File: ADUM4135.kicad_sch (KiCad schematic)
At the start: 24 parts

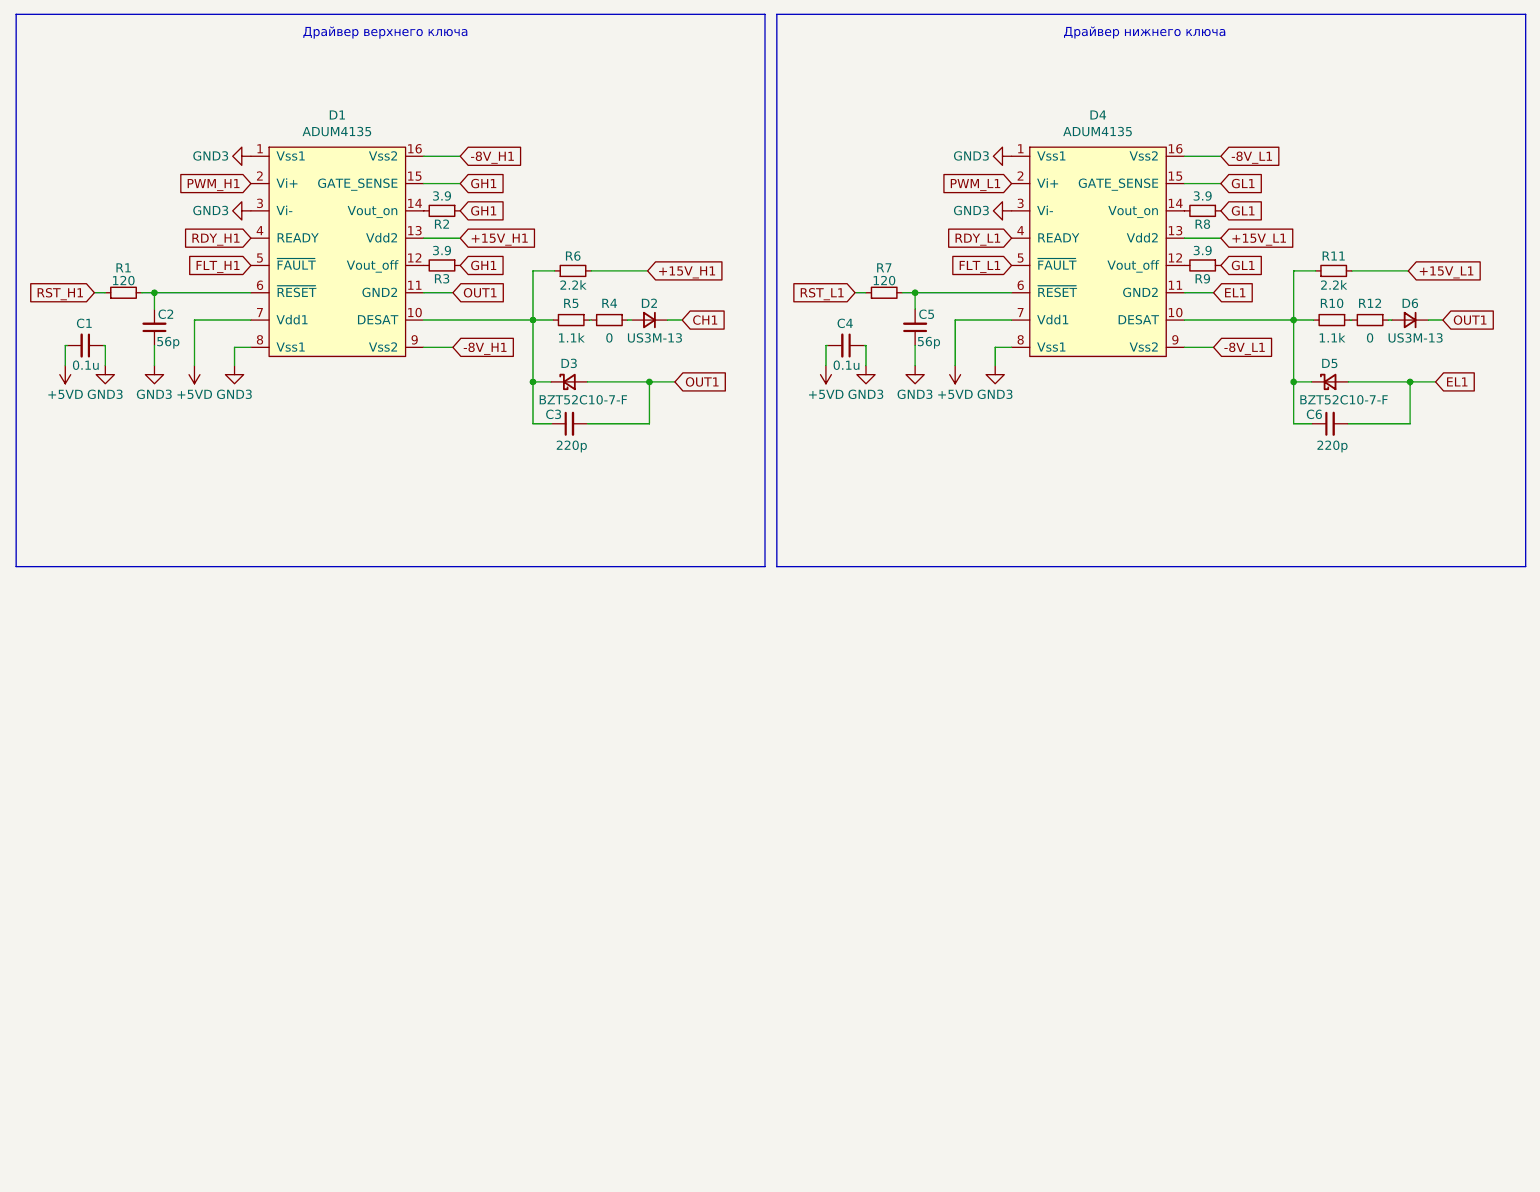
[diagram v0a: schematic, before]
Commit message: Одна стойка
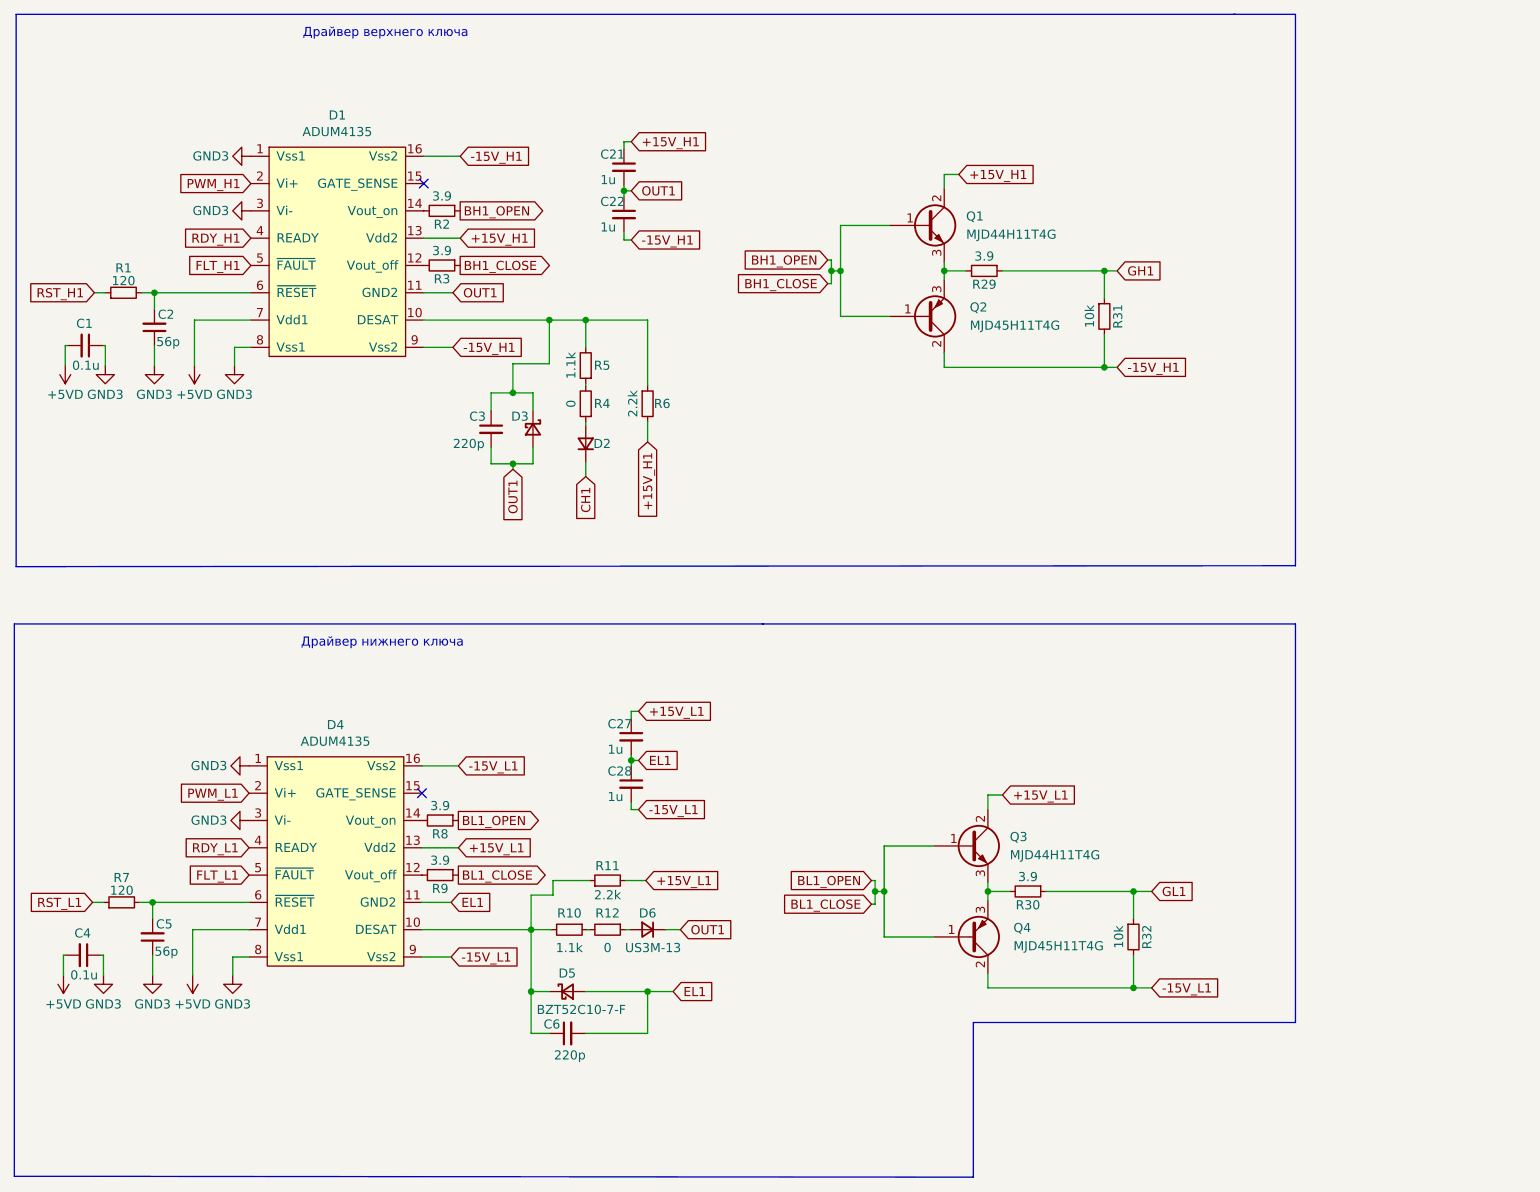
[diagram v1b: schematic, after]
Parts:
- added C21, C22, C27, C28: 1u, Capacitor_SMD:C_0805_2012Metric_Pad1.18x1.45mm_HandSolder, symbol Device:C_Small
- added Q1, Q3: MJD44H11T4G, Package_TO_SOT_SMD:TO-252-2, symbol Transistor_BJT:BCP56
- added Q2, Q4: MJD45H11T4G, Package_TO_SOT_SMD:TO-252-2, symbol Transistor_BJT:2SB817
- added R29, R30: 3.9, Resistor_SMD:R_2512_6332Metric_Pad1.40x3.35mm_HandSolder, symbol Device:R_Small
- added R31, R32: 10k, Resistor_SMD:R_2512_6332Metric_Pad1.40x3.35mm_HandSolder, symbol Device:R_Small
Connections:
- net +15V_H1: now also C21.1, Q1.2 (C), Q1.4 (C)
- net +15V_L1: now also C27.1, Q3.2 (C), Q3.4 (C)
- net EL1: now also C27.2, C28.1
- net GH1: now also R29.1, R31.1; no longer D1.15 (GATE_SENSE), R2.1, R3.1
- net GL1: now also R30.1, R32.1; no longer D4.15 (GATE_SENSE), R8.1, R9.1
- net OUT1: now also C21.2, C22.1
- net -8V_H1 renamed -15V_H1
- net -15V_H1: now also C22.2, Q2.2 (C), R31.2
- net -8V_L1 renamed -15V_L1
- net -15V_L1: now also C28.2, Q4.2 (C), R32.2
- new net: Q1.3 (E), Q2.3 (E), R29.2
- new net: Q3.3 (E), Q4.3 (E), R30.2
- new net BH1_CLOSE: Q1.1 (B), Q2.1 (B), R2.1, R3.1
- new net BL1_CLOSE: Q3.1 (B), Q4.1 (B), R8.1, R9.1
- no-connect marks 0 -> 2
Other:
- moved on the sheet: C3, C4, C5, C6, D2, D3, D4, D5, D6, R10, R11, R12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
